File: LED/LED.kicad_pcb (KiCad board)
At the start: 2 copper layers, 160 x 100 mm, 35 parts, among them J1 1715721, Q1 CSD18501Q5A, U1 OPA192IDR, U2 TSR1-2450E

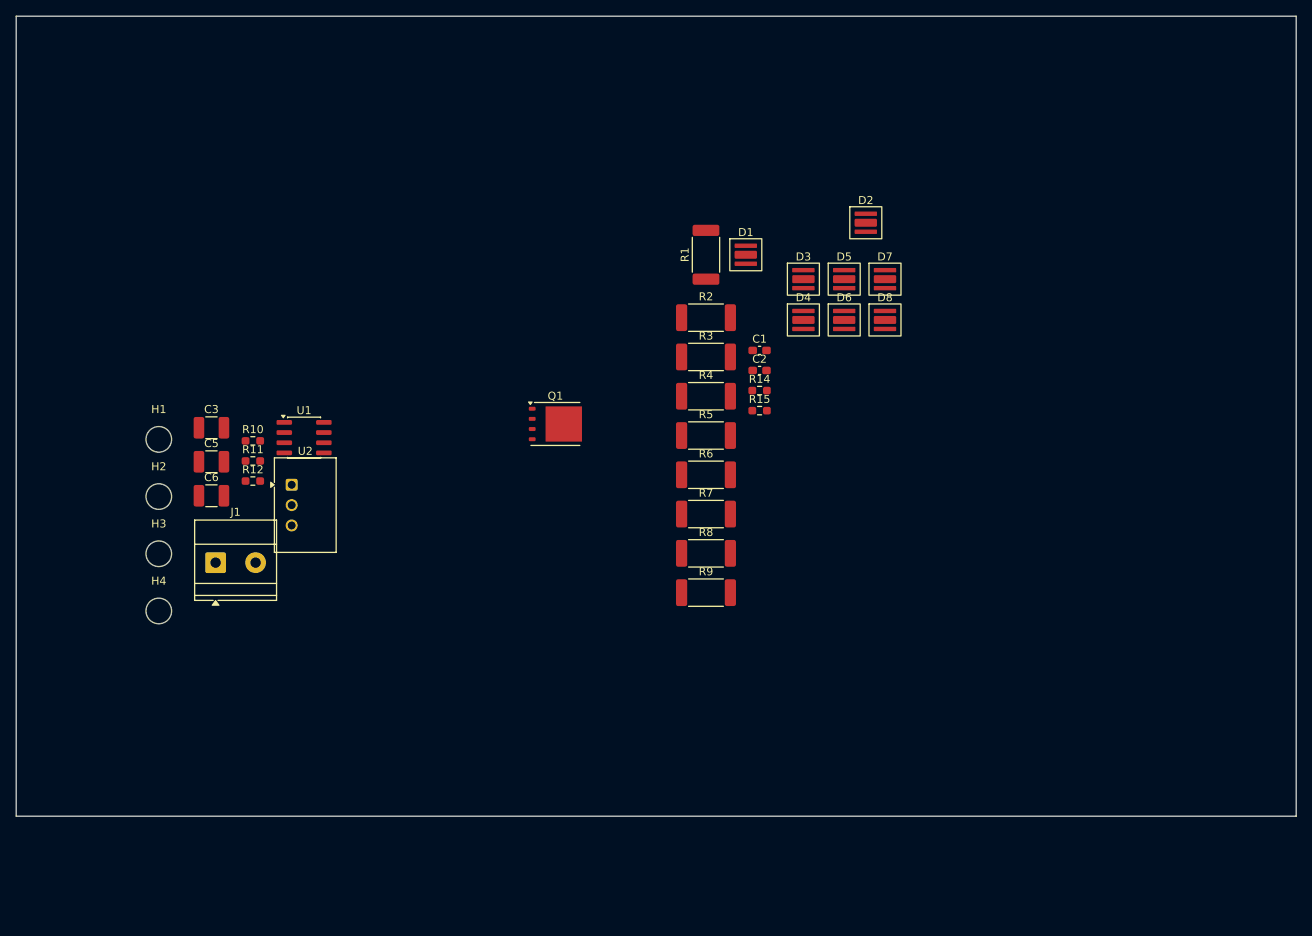
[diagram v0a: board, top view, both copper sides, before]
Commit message: Development
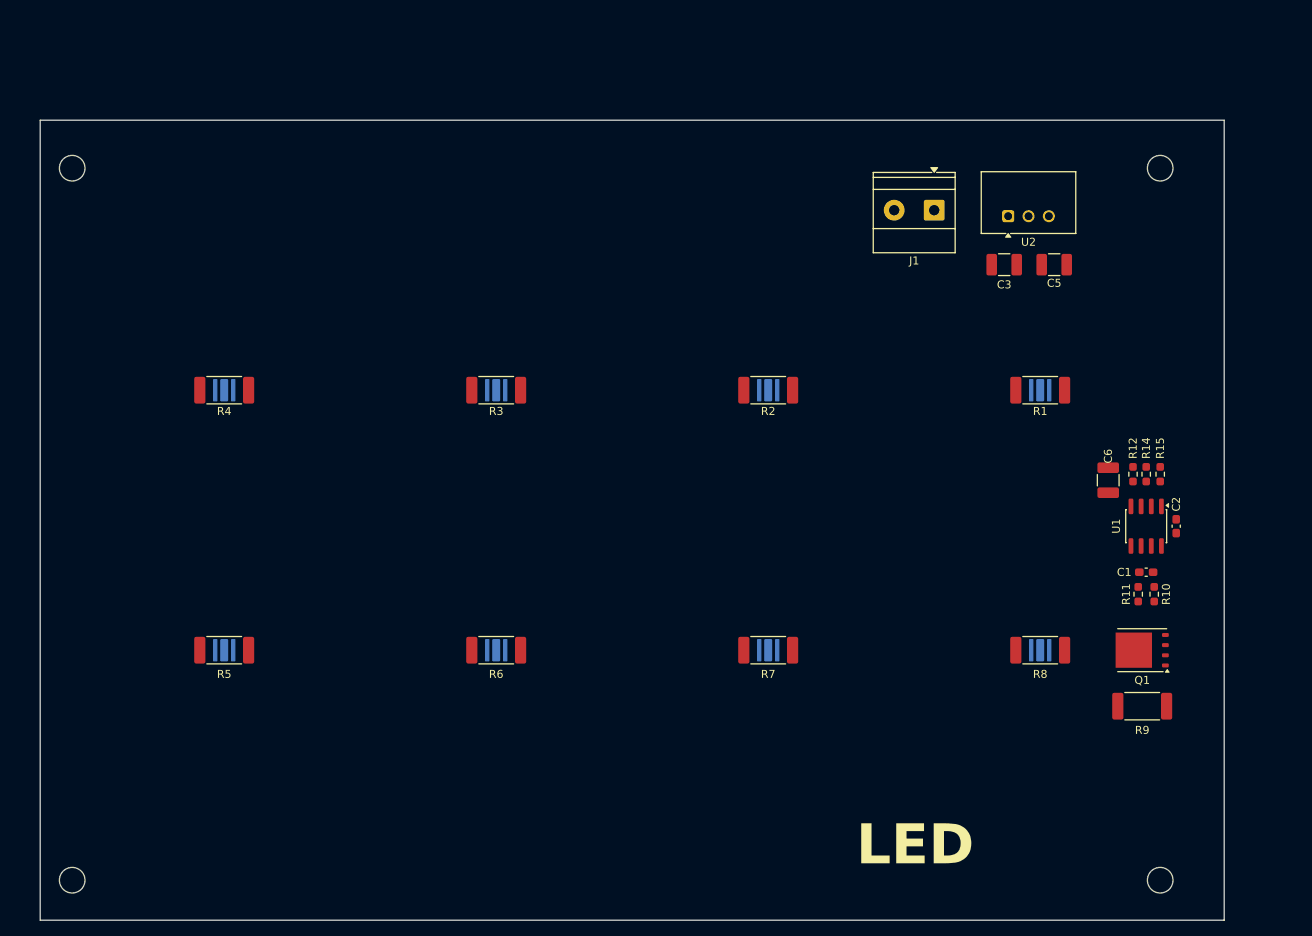
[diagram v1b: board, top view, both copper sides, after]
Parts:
- D1, D2, D3, D4, D5, D6, D7, D8: moved to B.Cu
- moved H3 134.1 mm to (213.0, 59.0)
- moved H4 129.6 mm to (213.0, 148.0)
- moved R10 114.3 mm to (212.2, 112.2), turned to -90 degrees
- moved C6 112.1 mm to (206.5, 98.0), turned to -90 degrees
- moved R11 111.9 mm to (210.2, 112.2), turned to -90 degrees
- moved R12 110.0 mm to (209.6, 97.2), turned to -90 degrees
- moved C5 108.2 mm to (199.8, 71.1), turned to 180 degrees
- moved U1 105.8 mm to (211.2, 103.8), turned to -90 degrees
- moved C3 101.2 mm to (193.5, 71.1)
- moved J1 100.0 mm to (184.8, 64.2), turned to 180 degrees
- moved U2 95.7 mm to (194.0, 65.0), turned to 90 degrees
- moved D5 90.3 mm to (96.0, 119.2), turned to 90 degrees
- moved Q1 78.6 mm to (210.8, 119.2), turned to 180 degrees
- moved D4 72.9 mm to (96.0, 86.8), turned to -90 degrees
- moved R5 65.9 mm to (96.0, 119.2)
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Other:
- board size 160 x 100 mm -> 148 x 100 mm
- board text added: "LED"
